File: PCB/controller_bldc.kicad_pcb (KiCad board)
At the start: 2 copper layers, 210 x 125 mm, 73 parts, among them J1 Battery Supply, J2 Conn_01x11_Male, J6 LM35, J7 Hall Sensors, J9 BLDC Motor, K1 RAYEX-L90B, Q1 IRF1010N, Q2 IRF1010N, Q3 IRF1010N, Q4 IRF1010N, Q5 IRF1010N, Q6 IRF1010N, Q7 PN2222A, SW1 ON_OFF, U1 ESP32-DEVKITC-32D, U2 MC1458P, U3 LM2596SOURCE_Pin2, U4 IR2103, U5 LM2596SOURCE, U8 IR2103, U9 IR2103

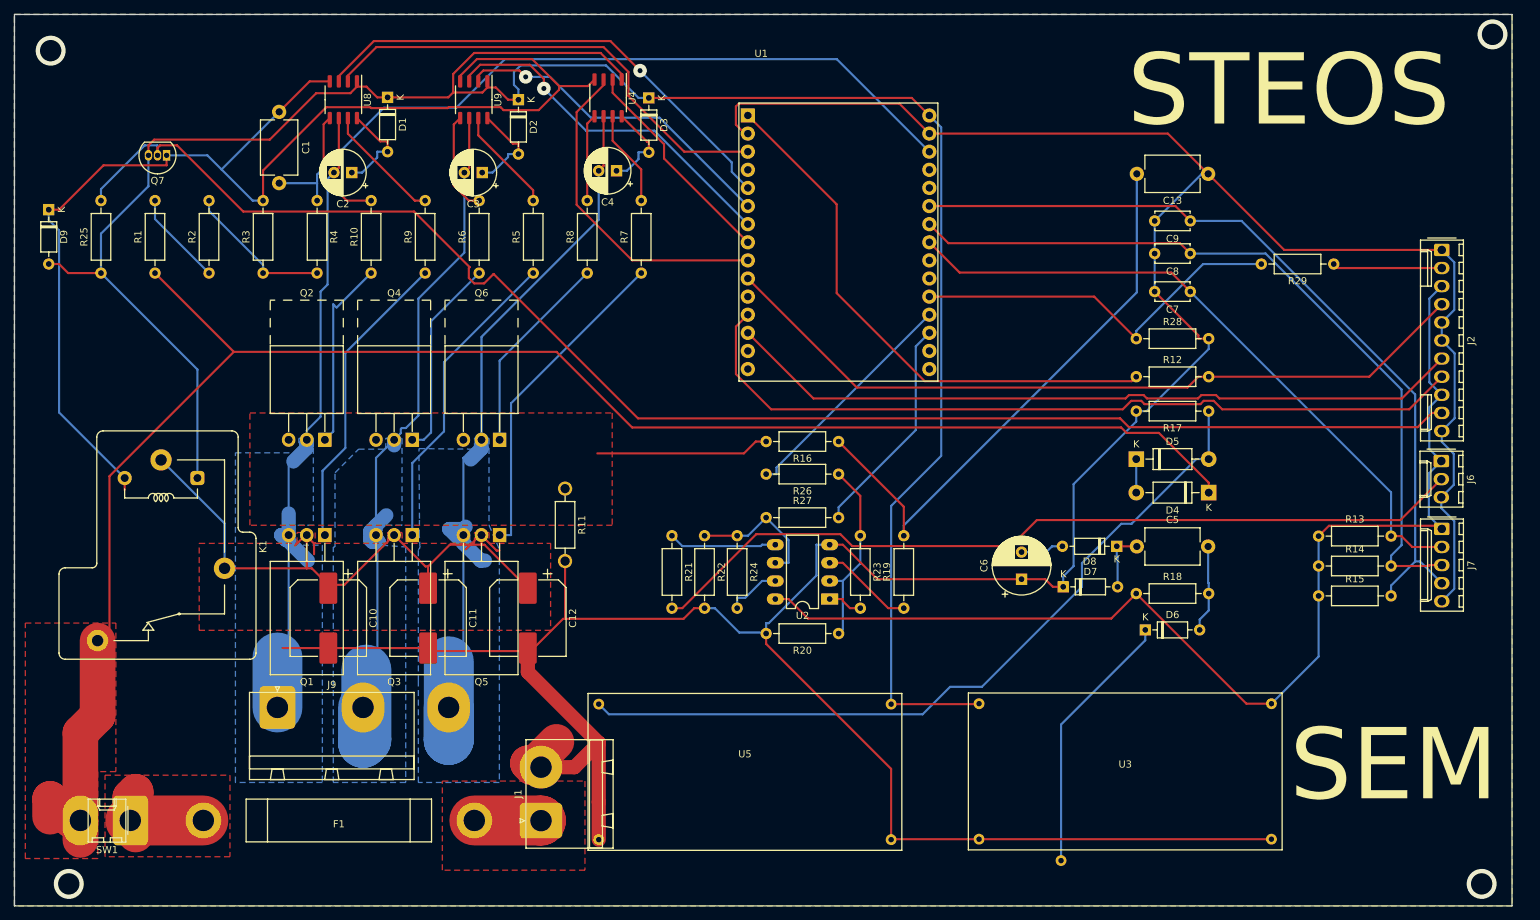
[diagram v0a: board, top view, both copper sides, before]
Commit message: Just before separating folders and branches According to version independence
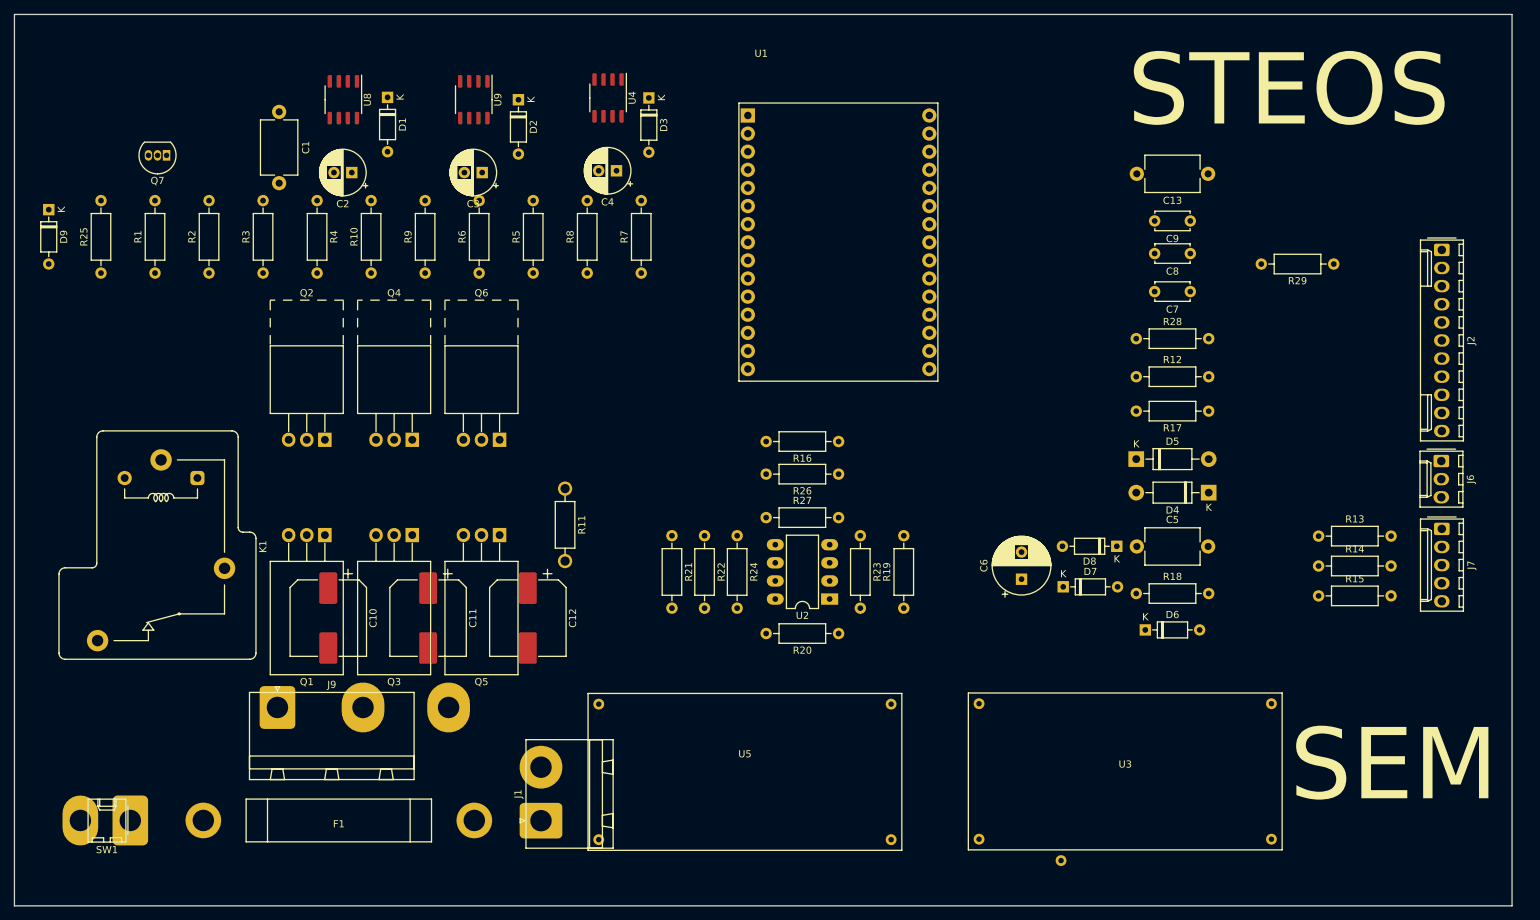
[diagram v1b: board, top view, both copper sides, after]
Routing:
- net GND: track 692.3 -> 0.00 mm, vias 4 -> 0
- net +12V: track 315.3 -> 0.00 mm
- net +36V: track 244.4 -> 0.00 mm
- net OPC_1: track 214.1 -> 0.00 mm
- net +5V: track 161.2 -> 0.00 mm
- net PH3: track 121.6 -> 0.00 mm
- net LM35-RAW: track 116.8 -> 0.00 mm
- net PH2: track 114.8 -> 0.00 mm
- net HALL-C: track 113.7 -> 0.00 mm
- net TX-LCD: track 113.3 -> 0.00 mm
- net Net-(D5-Pad2): track 109.6 -> 0.00 mm
- net Brake: track 108.5 -> 0.00 mm
- net HALL-B: track 108.4 -> 0.00 mm
- net Voltage_Sensor: track 106.9 -> 0.00 mm
- net RX-LCD: track 104.2 -> 0.00 mm
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- removed copper zone on F.Cu, net +36V
- removed copper zone on F.Cu, net 36V-Power
- removed copper zone on F.Cu, net Current_Sensor
- removed copper zone on B.Cu, net GND
- removed copper zone on F.Cu, net GND
- removed copper zone on F.Cu, net Net-(F1-Pad1)
- removed copper zone on F.Cu, net Net-(F1-Pad2)
- removed copper zone on B.Cu, net PH1
- removed copper zone on B.Cu, net PH2
- removed copper zone on B.Cu, net PH3
